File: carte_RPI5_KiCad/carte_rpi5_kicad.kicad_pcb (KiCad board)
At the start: 2 copper layers, 134.6 x 58.9 mm, 26 parts, among them J1 Conn_01x03, J10 RPI5_40pins, J2 Conn_01x03, J3 Conn_01x03, J4 Conn_01x03, J5 Conn_01x03, J6 Conn_01x03, J7 Conn_01x03, J8 Conn_01x03, J9 XT60-M, SW1 SW_SPDT

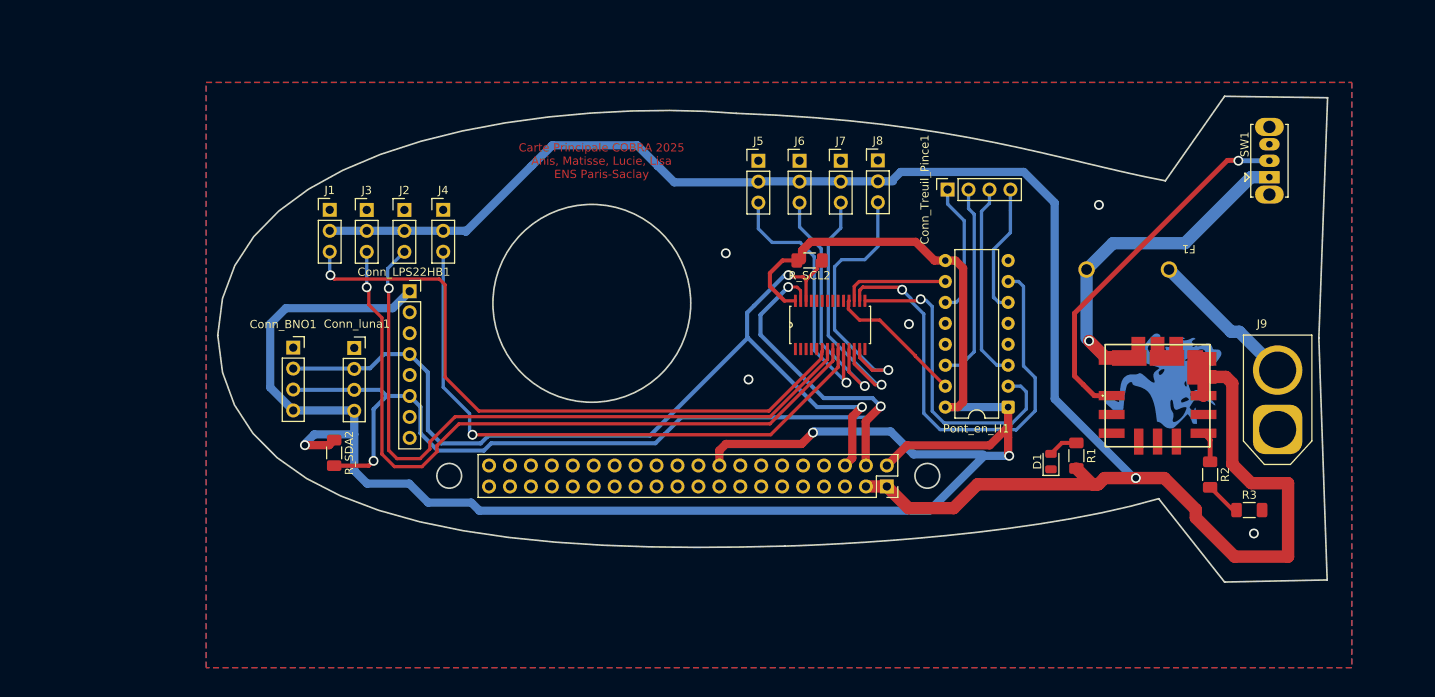
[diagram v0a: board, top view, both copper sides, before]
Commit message: maj carte
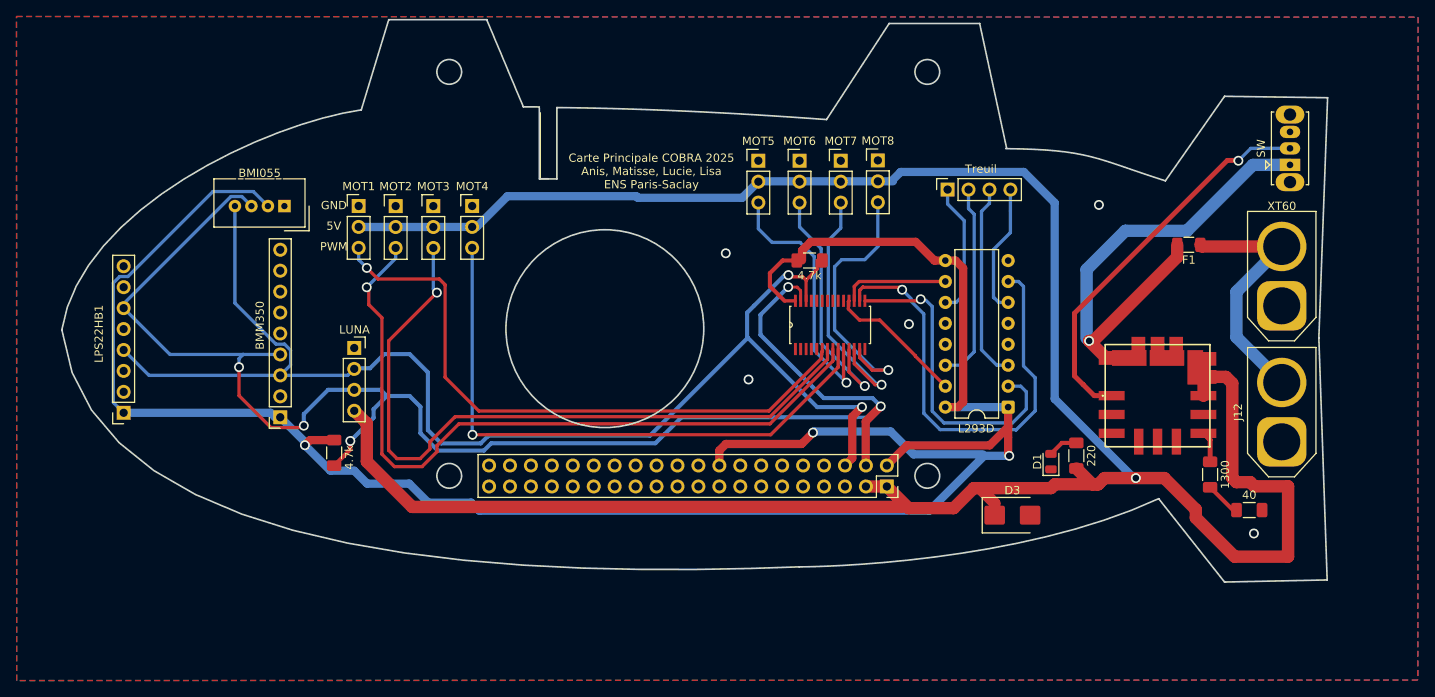
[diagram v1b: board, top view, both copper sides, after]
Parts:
- removed Conn_BNO1: Conn_01x04_Pin, Connector_PinSocket_2.54mm:PinSocket_1x04_P2.54mm_Vertical
- added BMI055: 110990030, Connector:NS-Tech_Grove_1x04_P2mm_Vertical, F.Cu at (70.5, 75.0)
- added BMM350: Conn_01x09_Pin, Connector_PinSocket_2.54mm:PinSocket_1x09_P2.54mm_Vertical, F.Cu at (70.0, 100.6)
- added D3: Z2SMBxxx, Diode_SMD:D_SMB, F.Cu at (158.8, 112.5)
- added J12: XT60-M, Connector_AMASS:AMASS_XT60-F_1x02_P7.20mm_Vertical, F.Cu at (191.5, 103.6)
- F1: footprint librairie_empreintes:PTF-50 -> Fuse:Fuse_1206_3216Metric
- moved LPS22HB1 37.7 mm to (51.0, 100.1), turned to 180 degrees
- moved XT60 15.0 mm to (191.5, 87.1)
- moved MOT1 3.54 mm to (79.5, 75.0)
- moved MOT2 3.54 mm to (84.0, 75.0)
- moved MOT4 3.54 mm to (93.3, 75.0)
- moved MOT3 3.54 mm to (88.6, 75.0)
- moved SW 2.92 mm to (192.5, 70.0)
- moved ? 1.21 mm to (179.4, 97.4)
- renumbered R2 to 1300, R1 to 220, R_SCL2 to 4.7k, R_SDA2 to 4.7k, R3 to 40, Pont_en_H1 to L293D, Conn_LPS22HB1 to LPS22HB1, Conn_luna1 to LUNA, J1 to MOT1, J3 to MOT2, J2 to MOT3, J4 to MOT4, J5 to MOT5, J6 to MOT6, J7 to MOT7, J8 to MOT8, SW1 to SW, Conn_Treuil_Pince1 to Treuil, J9 to XT60
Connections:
- LUNA pad 4: 3.3V -> 5V
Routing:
- net 5V: track 232.0 -> 304.0 mm
- net SDA: track 132.6 -> 185.4 mm, vias 3 -> 5
- net SCL: track 113.5 -> 160.2 mm
- net 3.3V: track 257.2 -> 277.2 mm
- net Net-(Régulateur_de_tension1-VIN): track 40.5 -> 60.0 mm
- net Net-(J12-POS): track 19.2 -> 31.0 mm
- net PWM0: track 79.5 -> 75.4 mm
- net Net-(Régulateur_de_tension1-ON/OFF_CONTROL): track 44.4 -> 47.5 mm
- net PWM1: track 85.4 -> 87.5 mm
- net PWM2: track 87.8 -> 89.8 mm
- net PWM3: track 74.1 -> 73.1 mm
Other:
- board size 134.6 x 58.9 mm -> 153.6 x 68.2 mm
- board text added: "5V"
- board text added: "GND"
- board text added: "PWM"
